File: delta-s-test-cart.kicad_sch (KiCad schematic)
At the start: 11 parts, among them J1 SNP, J2 ZXBUS, SW1 SW_DIP_x02, SW2 SW_Push, U1 74HCT32, U2 27C512

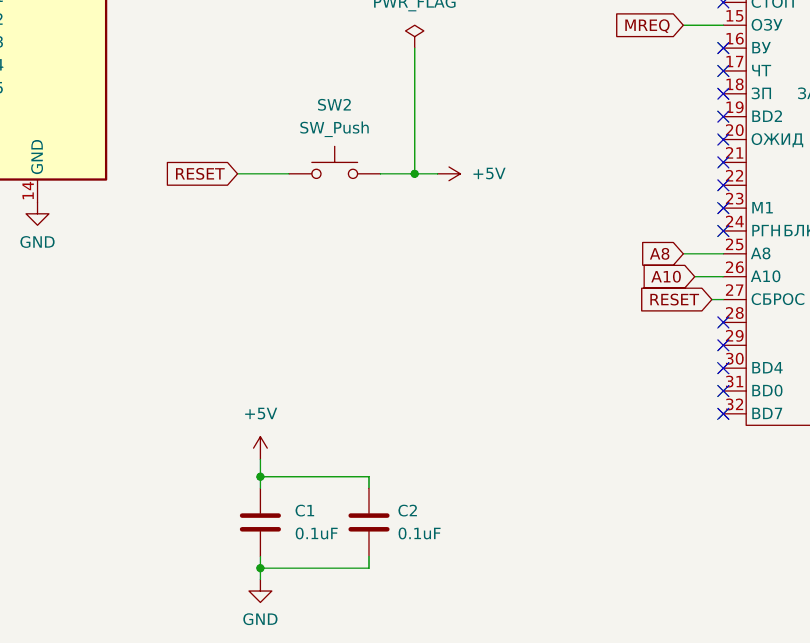
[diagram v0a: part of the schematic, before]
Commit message: Fixing stuff
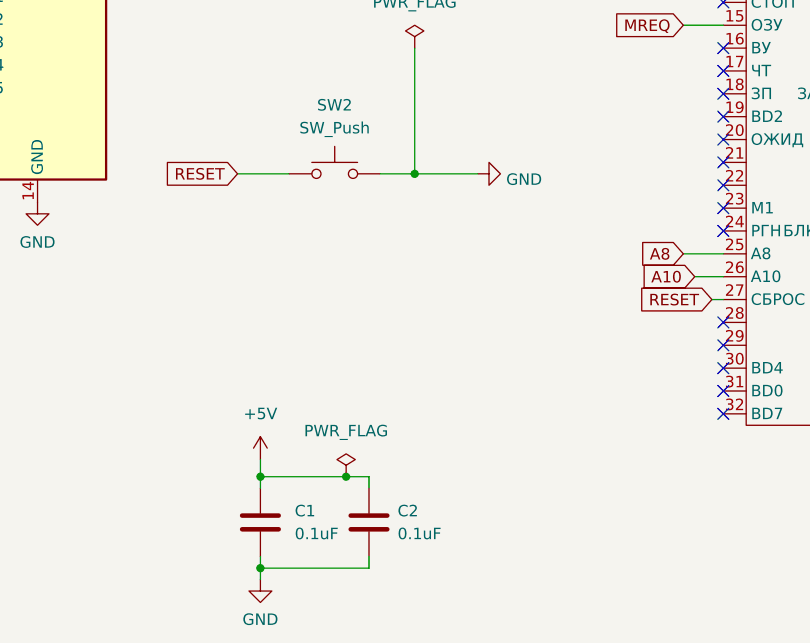
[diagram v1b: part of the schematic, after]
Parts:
- U2: footprint Package_DIP:DIP-28_W15.24mm -> Socket:DIP_Socket-28_W11.9_W12.7_W15.24_W17.78_W18.5_3M_228-1277-00-0602J
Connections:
- net +5V: no longer SW2.2
- net GND: now also SW2.2
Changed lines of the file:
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@@
   (junction (at 139.065 78.74) (diameter 0) (color 0 0 0 0)
+  )
+  (junction (at 131.445 112.395) (diameter 0) (color 0 0 0 0)
   )
   (junction (at 57.15 69.215) (diameter 0) (color 0 0 0 0)
@@
     (stroke (width 0) (type default))
   )
-  (wire (pts (xy 121.92 112.395) (xy 133.985 112.395))
+  (wire (pts (xy 121.92 112.395) (xy 131.445 112.395))
     (stroke (width 0) (type default))
   )
@@
     (stroke (width 0) (type default))
   )
+  (wire (pts (xy 131.445 112.395) (xy 133.985 112.395))
+    (stroke (width 0) (type default))
+  )
   (wire (pts (xy 241.935 95.25) (xy 238.125 95.25))
     (stroke (width 0) (type default))
@@
     (stroke (width 0) (type default))
   )
-  (wire (pts (xy 141.605 78.74) (xy 139.065 78.74))
+  (wire (pts (xy 146.05 78.74) (xy 139.065 78.74))
     (stroke (width 0) (type default))
   )
@@
     (pin "1")
     (instances
-      (project "zxcart"
+      (project "delta-s-test-cart"
         (path "/ecf6c71e-9caf-45b3-98d6-5b37bf48a9ce"
           (reference "#PWR0118") (unit 1)
@@
     (pin "2")
     (instances
-      (project "zxcart"
+      (project "delta-s-test-cart"
         (path "/ecf6c71e-9caf-45b3-98d6-5b37bf48a9ce"
           (reference "C2") (unit 1)
@@
     (pin "1")
     (instances
-      (project "zxcart"
+      (project "delta-s-test-cart"
         (path "/ecf6c71e-9caf-45b3-98d6-5b37bf48a9ce"
           (reference "#PWR0101") (unit 1)
@@
     (pin "9")
     (instances
-      (project "zxcart"
+      (project "delta-s-test-cart"
         (path "/ecf6c71e-9caf-45b3-98d6-5b37bf48a9ce"
           (reference "U1") (unit 1)
@@
     (pin "2")
     (instances
-      (project "zxcart"
+      (project "delta-s-test-cart"
         (path "/ecf6c71e-9caf-45b3-98d6-5b37bf48a9ce"
           (reference "SW2") (unit 1)
@@
     (pin "1")
     (instances
-      (project "zxcart"
+      (project "delta-s-test-cart"
         (path "/ecf6c71e-9caf-45b3-98d6-5b37bf48a9ce"
           (reference "#PWR0109") (unit 1)
@@
     (pin "9")
     (instances
-      (project "zxcart"
+      (project "delta-s-test-cart"
         (path "/ecf6c71e-9caf-45b3-98d6-5b37bf48a9ce"
           (reference "J2") (unit 1)
@@
     (pin "9")
     (instances
-      (project "zxcart"
+      (project "delta-s-test-cart"
         (path "/ecf6c71e-9caf-45b3-98d6-5b37bf48a9ce"
           (reference "J1") (unit 1)
@@
     (pin "1")
     (instances
-      (project "zxcart"
+      (project "delta-s-test-cart"
         (path "/ecf6c71e-9caf-45b3-98d6-5b37bf48a9ce"
           (reference "#PWR0108") (unit 1)
@@
     (pin "2")
     (instances
-      (project "zxcart"
+      (project "delta-s-test-cart"
         (path "/ecf6c71e-9caf-45b3-98d6-5b37bf48a9ce"
           (reference "R1") (unit 1)
@@
     (pin "1")
     (instances
-      (project "zxcart"
+      (project "delta-s-test-cart"
         (path "/ecf6c71e-9caf-45b3-98d6-5b37bf48a9ce"
           (reference "#PWR0105") (unit 1)
@@
     (pin "2")
     (instances
-      (project "zxcart"
+      (project "delta-s-test-cart"
         (path "/ecf6c71e-9caf-45b3-98d6-5b37bf48a9ce"
           (reference "R2") (unit 1)
@@
     (pin "1")
     (instances
-      (project "zxcart"
+      (project "delta-s-test-cart"
         (path "/ecf6c71e-9caf-45b3-98d6-5b37bf48a9ce"
           (reference "#FLG0102") (unit 1)
@@
     (pin "1")
     (instances
-      (project "zxcart"
+      (project "delta-s-test-cart"
         (path "/ecf6c71e-9caf-45b3-98d6-5b37bf48a9ce"
           (reference "#PWR0106") (unit 1)
@@
     )
   )
+  (symbol (lib_id "power:PWR_FLAG") (at 131.445 112.395 0) (unit 1)
+    (in_bom yes) (on_board yes) (dnp no) (fields_autoplaced)
+    (property "Reference" "#FLG01" (at 131.445 110.49 0)
+      (effects (font (size 1.27 1.27)) hide)
+    )
+    (property "Value" "PWR_FLAG" (at 131.445 107.315 0)
+      (effects (font (size 1.27 1.27)))
+    )
+    (property "Footprint" "" (at 131.445 112.395 0)
+      (effects (font (size 1.27 1.27)) hide)
+    )
+    (property "Datasheet" "~" (at 131.445 112.395 0)
+      (effects (font (size 1.27 1.27)) hide)
+    )
+    (pin "1")
+    (instances
+      (project "delta-s-test-cart"
+        (path "/ecf6c71e-9caf-45b3-98d6-5b37bf48a9ce"
+          (reference "#FLG01") (unit 1)
+        )
+      )
+    )
+  )
   (symbol (lib_id "power:PWR_FLAG") (at 139.065 64.77 0) (unit 1)
     (in_bom yes) (on_board yes) (dnp no) (fields_autoplaced)
@@
     (pin "1")
     (instances
-      (project "zxcart"
+      (project "delta-s-test-cart"
         (path "/ecf6c71e-9caf-45b3-98d6-5b37bf48a9ce"
           (reference "#FLG0101") (unit 1)
+        )
+      )
+    )
+  )
+  (symbol (lib_id "power:GND") (at 146.05 78.74 90) (unit 1)
+    (in_bom yes) (on_board yes) (dnp no) (fields_autoplaced)
+    (property "Reference" "#PWR01" (at 152.4 78.74 0)
+      (effects (font (size 1.27 1.27)) hide)
+    )
+    (property "Value" "GND" (at 149.225 79.375 90)
+      (effects (font (size 1.27 1.27)) (justify right))
+    )
+    (property "Footprint" "" (at 146.05 78.74 0)
+      (effects (font (size 1.27 1.27)) hide)
+    )
+    (property "Datasheet" "" (at 146.05 78.74 0)
+      (effects (font (size 1.27 1.27)) hide)
+    )
+    (pin "1")
+    (instances
+      (project "delta-s-test-cart"
+        (path "/ecf6c71e-9caf-45b3-98d6-5b37bf48a9ce"
+          (reference "#PWR01") (unit 1)
         )
       )
@@
     (pin "2")
     (instances
-      (project "zxcart"
+      (project "delta-s-test-cart"
         (path "/ecf6c71e-9caf-45b3-98d6-5b37bf48a9ce"
           (reference "R3") (unit 1)
@@
     (pin "1")
     (instances
-      (project "zxcart"
+      (project "delta-s-test-cart"
         (path "/ecf6c71e-9caf-45b3-98d6-5b37bf48a9ce"
           (reference "#PWR0119") (unit 1)
@@
     (pin "1")
     (instances
-      (project "zxcart"
+      (project "delta-s-test-cart"
         (path "/ecf6c71e-9caf-45b3-98d6-5b37bf48a9ce"
           (reference "#PWR0110") (unit 1)
@@
     (pin "1")
     (instances
-      (project "zxcart"
+      (project "delta-s-test-cart"
         (path "/ecf6c71e-9caf-45b3-98d6-5b37bf48a9ce"
           (reference "#PWR0114") (unit 1)
@@
     (pin "4")
     (instances
-      (project "zxcart"
+      (project "delta-s-test-cart"
         (path "/ecf6c71e-9caf-45b3-98d6-5b37bf48a9ce"
           (reference "SW1") (unit 1)
@@
     (pin "1")
     (instances
-      (project "zxcart"
+      (project "delta-s-test-cart"
         (path "/ecf6c71e-9caf-45b3-98d6-5b37bf48a9ce"
           (reference "#PWR0107") (unit 1)
-        )
-      )
-    )
-  )
-  (symbol (lib_id "power:+5V") (at 141.605 78.74 270) (unit 1)
-    (in_bom yes) (on_board yes) (dnp no) (fields_autoplaced)
-    (property "Reference" "#PWR0116" (at 137.795 78.74 0)
-      (effects (font (size 1.27 1.27)) hide)
-    )
-    (property "Value" "+5V" (at 145.415 78.7399 90)
-      (effects (font (size 1.27 1.27)) (justify left))
-    )
-    (property "Footprint" "" (at 141.605 78.74 0)
-      (effects (font (size 1.27 1.27)) hide)
-    )
-    (property "Datasheet" "" (at 141.605 78.74 0)
-      (effects (font (size 1.27 1.27)) hide)
-    )
-    (pin "1")
-    (instances
-      (project "zxcart"
-        (path "/ecf6c71e-9caf-45b3-98d6-5b37bf48a9ce"
-          (reference "#PWR0116") (unit 1)
         )
       )
@@
     (pin "1")
     (instances
-      (project "zxcart"
+      (project "delta-s-test-cart"
         (path "/ecf6c71e-9caf-45b3-98d6-5b37bf48a9ce"
           (reference "#PWR0117") (unit 1)
@@
     (pin "1")
     (instances
-      (project "zxcart"
+      (project "delta-s-test-cart"
         (path "/ecf6c71e-9caf-45b3-98d6-5b37bf48a9ce"
           (reference "#PWR0111") (unit 1)
@@
     (pin "2")
     (instances
-      (project "zxcart"
+      (project "delta-s-test-cart"
         (path "/ecf6c71e-9caf-45b3-98d6-5b37bf48a9ce"
           (reference "C1") (unit 1)
@@
     (pin "1")
     (instances
-      (project "zxcart"
+      (project "delta-s-test-cart"
         (path "/ecf6c71e-9caf-45b3-98d6-5b37bf48a9ce"
           (reference "#PWR0103") (unit 1)
@@
     (pin "1")
     (instances
-      (project "zxcart"
+      (project "delta-s-test-cart"
         (path "/ecf6c71e-9caf-45b3-98d6-5b37bf48a9ce"
           (reference "#PWR0102") (unit 1)
@@
     (pin "1")
     (instances
-      (project "zxcart"
+      (project "delta-s-test-cart"
         (path "/ecf6c71e-9caf-45b3-98d6-5b37bf48a9ce"
           (reference "#PWR0113") (unit 1)
@@
     (pin "1")
     (instances
-      (project "zxcart"
+      (project "delta-s-test-cart"
         (path "/ecf6c71e-9caf-45b3-98d6-5b37bf48a9ce"
           (reference "#PWR0115") (unit 1)
@@
       (effects (font (size 1.27 1.27)) (justify left))
     )
-    (property "Footprint" "Package_DIP:DIP-28_W15.24mm" (at 97.155 53.975 0)
+    (property "Footprint" "Socket:DIP_Socket-28_W11.9_W12.7_W15.24_W17.78_W18.5_3M_228-1277-00-0602J" (at 97.155 53.975 0)
       (effects (font (size 1.27 1.27)) hide)
     )
@@
     (pin "9")
     (instances
-      (project "zxcart"
+      (project "delta-s-test-cart"
         (path "/ecf6c71e-9caf-45b3-98d6-5b37bf48a9ce"
           (reference "U2") (unit 1)
@@
     (pin "1")
     (instances
-      (project "zxcart"
+      (project "delta-s-test-cart"
         (path "/ecf6c71e-9caf-45b3-98d6-5b37bf48a9ce"
           (reference "#PWR0112") (unit 1)
@@
     (pin "1")
     (instances
-      (project "zxcart"
+      (project "delta-s-test-cart"
         (path "/ecf6c71e-9caf-45b3-98d6-5b37bf48a9ce"
           (reference "#PWR0104") (unit 1)
